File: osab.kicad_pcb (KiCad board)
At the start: 2 copper layers, 50 x 75 mm, 98 parts, among them CON1 TF-01A, CON2 PJ-3420-A-SMT, CON3 TYPE-C-31-M-12, Q1 BC847B, Q2 BC847B, SW1 PPP, SW10 RESET, SW11 Torch, SW2 VOL-, SW3 VOL+, SW4 CHAP-, SW5 CHAP+, SW6 OT/NT, SW7 BOOK-, SW8 BOOK+, SW9 XKB5858-Z-F, U1 VS1000, U2 ME6211C33M5G-N, U3 CAT25640, U4 TP4055, U5 MF5853CS, U6 PAM8302AAS, Y1 12MHz

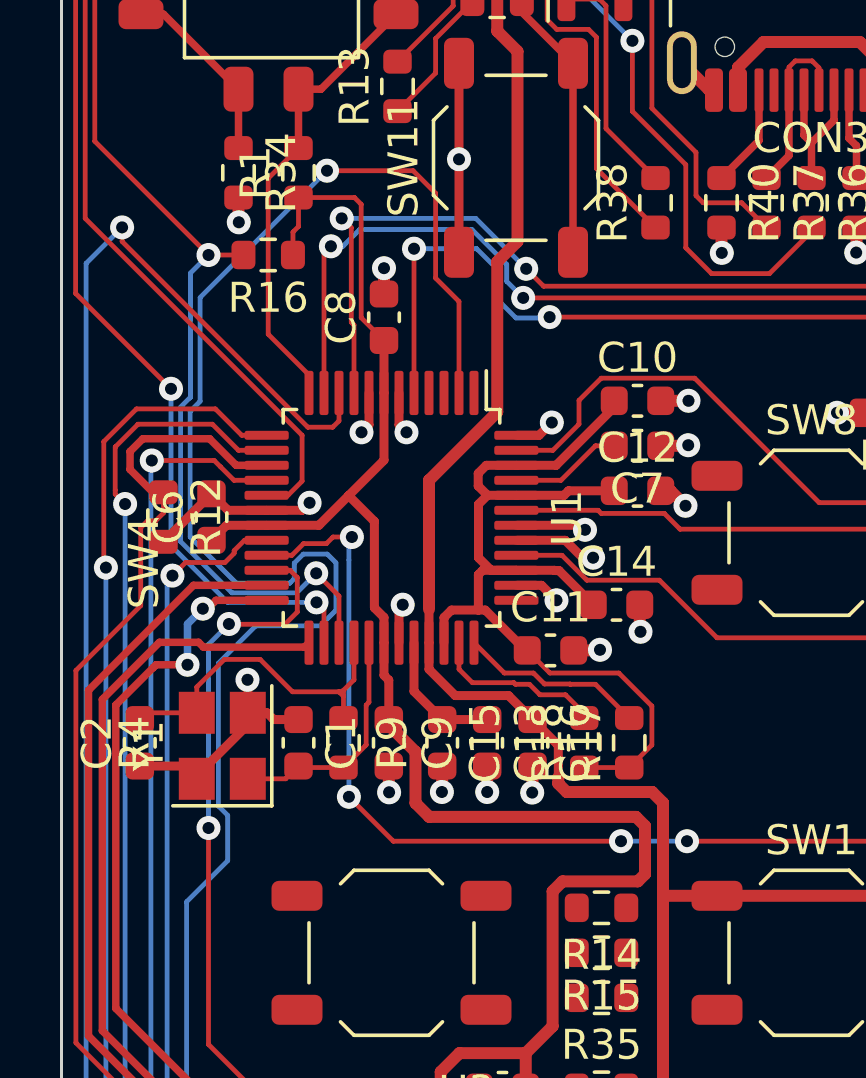
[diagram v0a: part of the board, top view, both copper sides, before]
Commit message: production: Routing tracks...
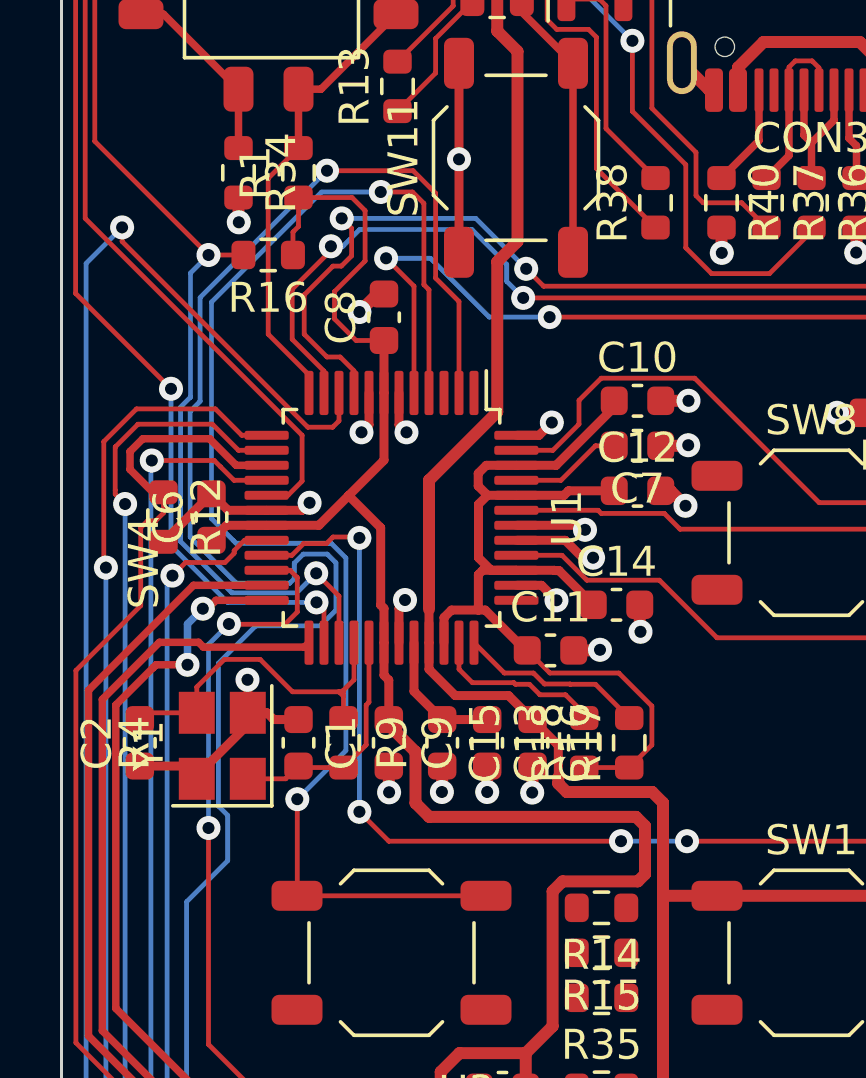
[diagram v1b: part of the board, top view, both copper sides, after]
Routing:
- net Net-(R4-Pad1): track 0.00 -> 45.6 mm, vias 0 -> 2
- net Net-(R6-Pad1): track 50.1 -> 51.9 mm
- net VDD: track 107.2 -> 108.5 mm
- net Net-(R8-Pad1): track 31.6 -> 32.5 mm
